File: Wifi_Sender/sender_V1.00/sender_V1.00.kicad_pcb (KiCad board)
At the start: 2 copper layers, 83.3 x 54.9 mm, 18 parts, among them J1 9-12V In, J10 Door_Closed, J2 9-12V Out, J3 I2C_1, J4 Motor_2, J5 Motor_1, J6 I2C_2, J7 Light Sensor, J8 I2C_3, J9 Door_Open, SW1 PowerSwitch, U1 ESP32-DEVKIT-V1

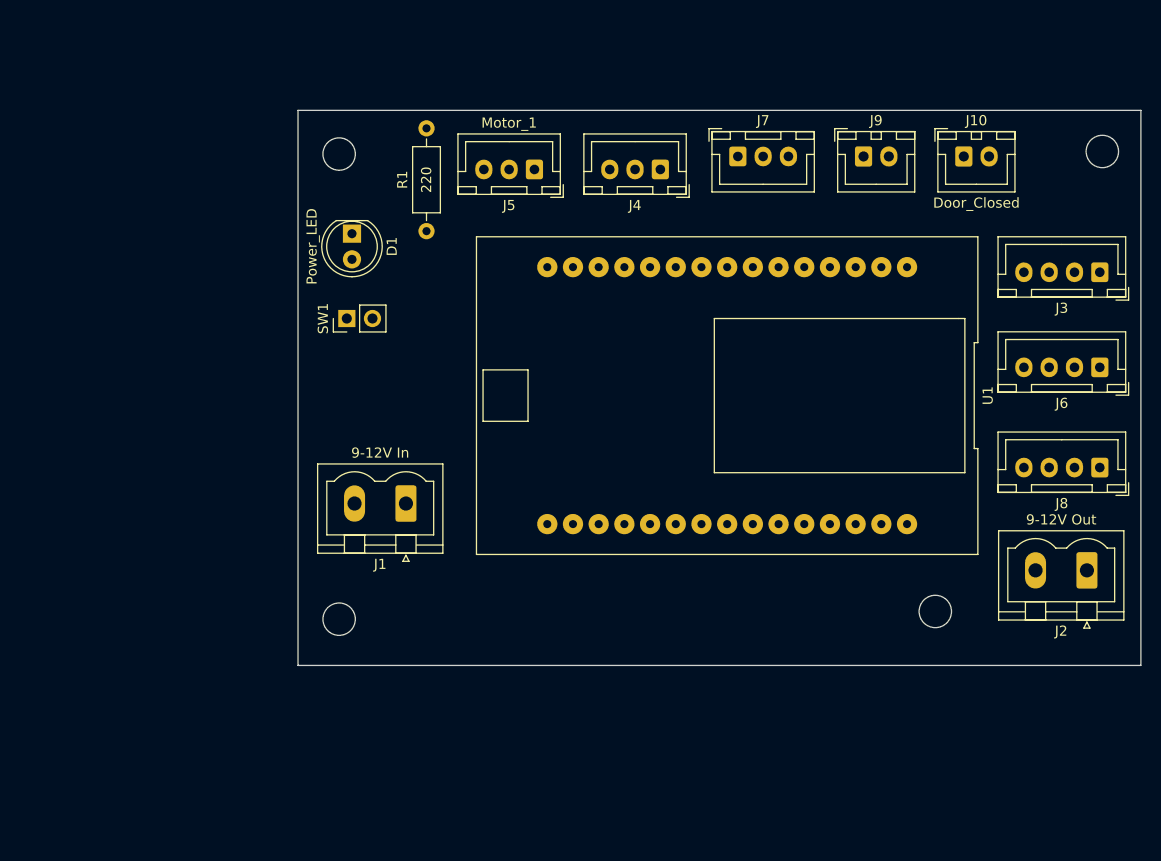
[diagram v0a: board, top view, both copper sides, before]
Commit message: Update
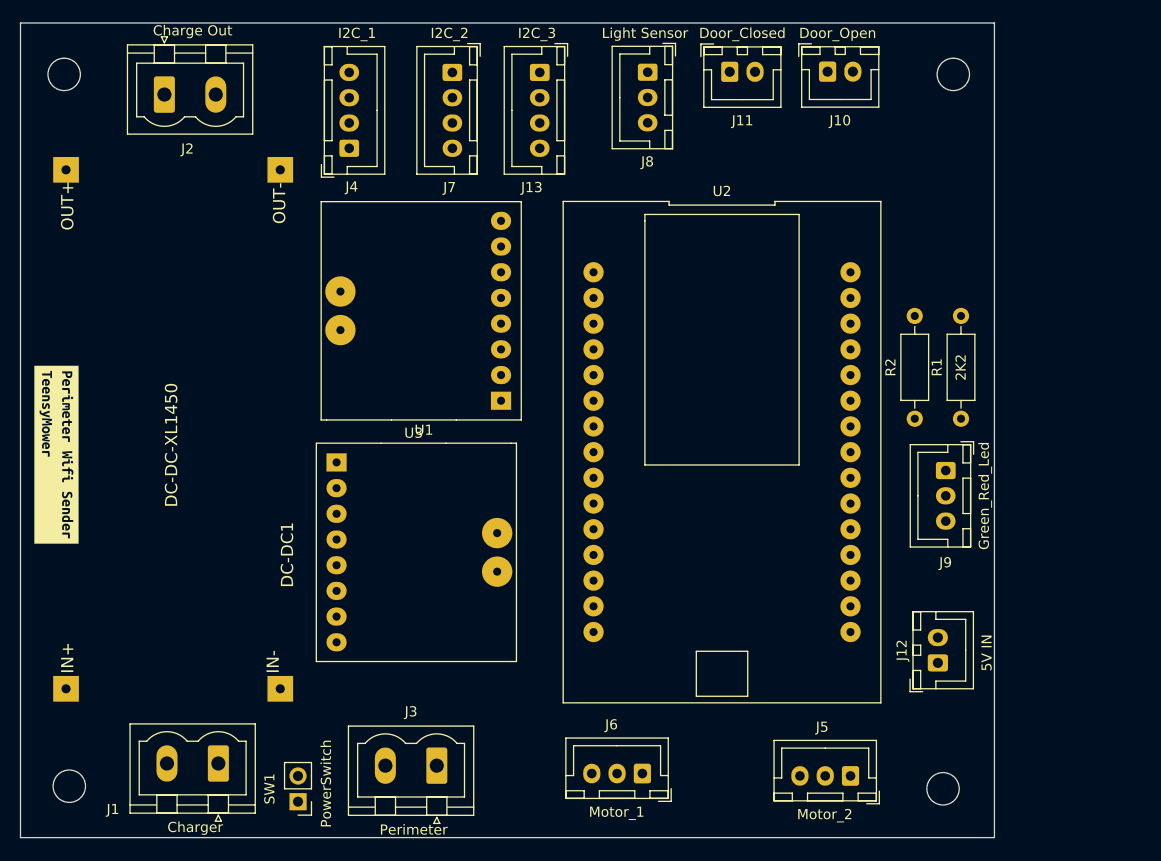
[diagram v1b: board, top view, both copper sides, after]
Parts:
- removed D1: Power_LED, LED_THT:LED_D5.0mm
- added DC-DC1: DC-DC-XL1450, Zimprich:DCDC-XL1450, F.Cu at (50.8, 61.0)
- added J11: Door_Closed, Connector_JST:JST_XH_B2B-XH-A_1x02_P2.50mm_Vertical, F.Cu at (103.9, 17.5)
- added J12: 5V IN, Connector_JST:JST_XH_B2B-XH-A_1x02_P2.50mm_Vertical, F.Cu at (124.5, 75.9)
- added J13: I2C_3, Connector_JST:JST_XH_B4B-XH-A_1x04_P2.50mm_Vertical, F.Cu at (85.1, 17.6)
- added R2: 220, Resistor_THT:R_Axial_DIN0207_L6.3mm_D2.5mm_P10.16mm_Horizontal, F.Cu at (122.2, 51.8)
- added U2: ESP32-DEVKIT-V1, teensy_library-master:ESP32-DEVKIT-V1, F.Cu at (103.1, 55.1)
- added U3: INA226-Sense_I2C, Current_sense:INA226, F.Cu at (72.6, 65.0)
- added kibuzzard-63696024: G***, kibuzzard-63696024, F.Cu at (37.3, 55.4)
- J1: value 9-12V In -> Charger
- J10: value Door_Closed -> Door_Open
- J2: value 9-12V Out -> Charge Out
- J3: value I2C_1 -> Perimeter; footprint Connector_JST:JST_XH_B4B-XH-A_1x04_P2.50mm_Vertical -> Connector_Phoenix_MSTB:PhoenixContact_MSTBVA_2,5_2-G-5,08_1x02_P5.08mm_Vertical
- J4: value Motor_2 -> I2C_1; footprint Connector_JST:JST_XH_B3B-XH-A_1x03_P2.50mm_Vertical -> Connector_JST:JST_XH_B4B-XH-A_1x04_P2.50mm_Vertical
- J5: value Motor_1 -> Motor_2
- J6: value I2C_2 -> Motor_1; footprint Connector_JST:JST_XH_B4B-XH-A_1x04_P2.50mm_Vertical -> Connector_JST:JST_XH_B3B-XH-A_1x03_P2.50mm_Vertical
- J7: value Light Sensor -> I2C_2; footprint Connector_JST:JST_XH_B3B-XH-A_1x03_P2.50mm_Vertical -> Connector_JST:JST_XH_B4B-XH-A_1x04_P2.50mm_Vertical
- J8: value I2C_3 -> Light Sensor; footprint Connector_JST:JST_XH_B4B-XH-A_1x04_P2.50mm_Vertical -> Connector_JST:JST_XH_B3B-XH-A_1x03_P2.50mm_Vertical
- J9: value Door_Open -> Green_Red_Led; footprint Connector_JST:JST_XH_B2B-XH-A_1x02_P2.50mm_Vertical -> Connector_JST:JST_XH_B3B-XH-A_1x03_P2.50mm_Vertical
- R1: value 220 -> 2K2
- U1: value ESP32-DEVKIT-V1 -> INA226-Sense_I2C; footprint teensy_library-master:ESP32-DEVKIT-V1 -> Current_sense:INA226
- moved J2 102.6 mm to (48.0, 19.8), turned to 0 degrees
- moved J3 81.7 mm to (74.9, 86.1)
- moved J5 67.6 mm to (115.8, 87.1)
- moved H1 64.9 mm to (125.0, 88.4)
- moved J6 60.5 mm to (95.2, 86.9)
- moved J8 59.4 mm to (95.8, 17.6), turned to -90 degrees
- moved R1 56.0 mm to (126.7, 51.8)
- moved H3 53.1 mm to (126.0, 17.8)
- moved SW1 48.0 mm to (61.2, 89.7), turned to 180 degrees
- moved J9 32.1 mm to (125.2, 56.9), turned to -90 degrees
- moved J1 31.7 mm to (53.3, 85.9)
- moved H2 31.4 mm to (38.6, 88.1)
- moved U1 31.1 mm to (73.7, 41.1), turned to 90 degrees
- moved J4 30.8 mm to (66.3, 25.1), turned to 90 degrees
- moved J7 29.4 mm to (76.5, 17.6), turned to -90 degrees
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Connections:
- J10 pad 2: Door_Closed -> Door_Open
- J3 pad 1: SDA -> Net-(J3-Pad1)
- J3 pad 2: SCL -> GND
- J4 pad 1: Enable_B -> SDA
- J4 pad 2: Input_4 -> SCL
- J4 pad 3: Input_3 -> GND
- J5 pad 1: Enable_A -> Enable_B
- J5 pad 2: Input_1 -> Input_4
- J5 pad 3: Input_2 -> Input_3
- J6 pad 1: SDA -> Enable_A
- J6 pad 2: SCL -> Input_1
- J6 pad 3: GND -> Input_2
- J7 pad 1: +3V3 -> SDA
- J7 pad 2: GND -> SCL
- J7 pad 3: D0 -> GND
- J8 pad 1: SDA -> +3V3
- J8 pad 2: SCL -> GND
- J8 pad 3: GND -> D0
- J9 pad 2: Door_Open -> Net-(J9-Pad2)
- R1 pad 1: Net-(D1-Pad2) -> Net-(J9-Pad2)
- R1 pad 2: +3V3 -> RED
- SW1 pad 2: Net-(J2-Pad1) -> Net-(DC-DC1-PadI+)
- U1 pad 10: unconnected-(U1-Pad10) -> Net-(J2-Pad1)
- U1 pad 3: unconnected-(U1-Pad3) -> Net-(DC-DC1-PadI+)
- U1 pad 5: D0 -> SCL
- U1 pad 6: unconnected-(U1-Pad6) -> SDA
- U1 pad 7: unconnected-(U1-Pad7) -> GND
- U1 pad 8: unconnected-(U1-Pad8) -> +3V3
- U1 pad 9: unconnected-(U1-Pad9) -> Net-(DC-DC1-PadI+)
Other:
- board size 83.3 x 54.9 mm -> 96.3 x 80.5 mm
